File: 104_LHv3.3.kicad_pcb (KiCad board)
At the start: 2 copper layers, 437.8 x 130.6 mm, 241 parts, among them K1 CHRY_MX, K10 CHRY_MX, K100 CHRY_MX, K101 CHRY_MX, K102 CHRY_MX, K103 CHRY_MX, K104 CHRY_MX, K11 CHRY_MX, K12 CHRY_MX, K13 CHRY_MX, K14 CHRY_MX, K15 CHRY_MX, K16 CHRY_MX, K17 CHRY_MX, K18 CHRY_MX, K19 CHRY_MX, K2 CHRY_MX, K20 CHRY_MX, K21 CHRY_MX, K22 CHRY_MX, K23 CHRY_MX, K24 CHRY_MX, K25 CHRY_MX, K26 CHRY_MX, K27 CHRY_MX, K28 CHRY_MX, K29 CHRY_MX, K3 CHRY_MX, K30 CHRY_MX, K31 CHRY_MX, K32 CHRY_MX, K33 CHRY_MX, K34 CHRY_MX, K35 CHRY_MX, K36 CHRY_MX, K37 CHRY_MX, K38 CHRY_MX, K39 CHRY_MX, K4 CHRY_MX, K40 CHRY_MX, K41 CHRY_MX, K42 CHRY_MX, K43 CHRY_MX, K44 CHRY_MX, K45 CHRY_MX, K46 CHRY_MX, K47 CHRY_MX, K48 CHRY_MX, K49 CHRY_MX, K5 CHRY_MX, K50 CHRY_MX, K51 CHRY_MX, K52 CHRY_MX, K53 CHRY_MX, K54 CHRY_MX, K55 CHRY_MX, K56 CHRY_MX, K57 CHRY_MX, K58 CHRY_MX, K59 CHRY_MX, K6 CHRY_MX, K60 CHRY_MX, K61 CHRY_MX, K62 CHRY_MX, K63 CHRY_MX, K64 CHRY_MX, K65 CHRY_MX, K66 CHRY_MX, K67 CHRY_MX, K68 CHRY_MX, K69 CHRY_MX, K7 CHRY_MX, K70 CHRY_MX, K71 CHRY_MX, K72 CHRY_MX, K73 CHRY_MX, K74 CHRY_MX, K75 CHRY_MX, K76 CHRY_MX, K77 CHRY_MX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

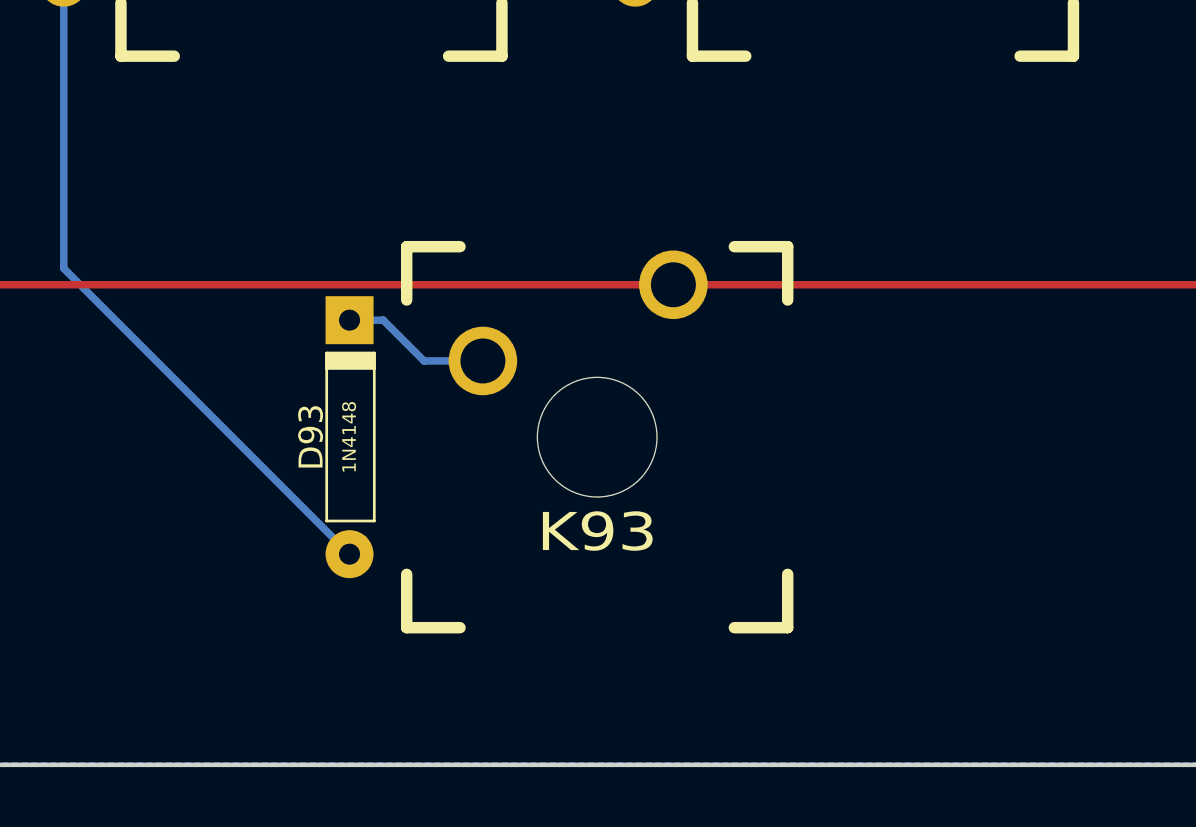
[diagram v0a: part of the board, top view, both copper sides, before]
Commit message: Tweaks in Stabs
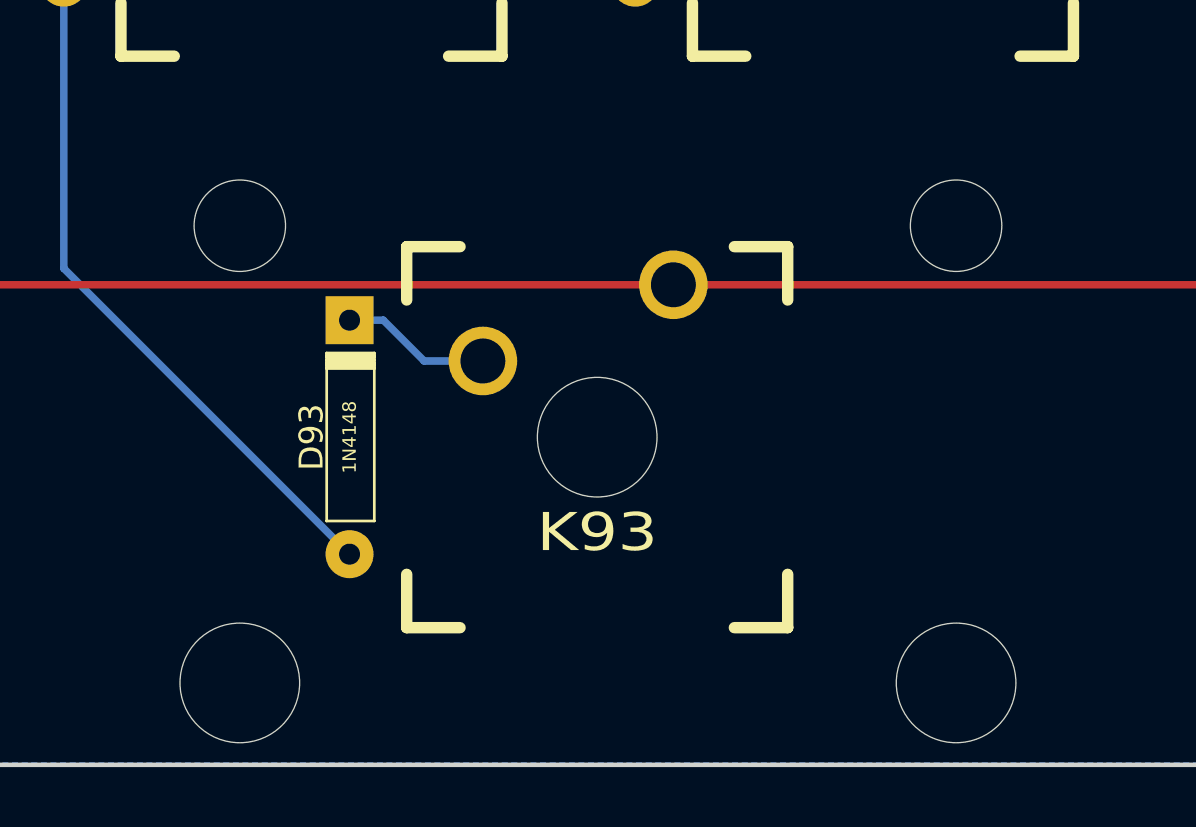
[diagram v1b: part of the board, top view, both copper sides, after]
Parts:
- added 2.0u: 2.0u, mx_stabs:Mx_Stab_200, F.Cu at (116.2, 197.4)
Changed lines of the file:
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@@
     (tracks 1560)
     (zones 0)
-    (modules 241)
+    (modules 242)
     (nets 159)
   )
@@
     (add_net /VCC)
   )
+  (module mx_stabs:Mx_Stab_200 (layer F.Cu)
+    (at 116.2304 197.4215)
+    (descr MXALPS)
+    (tags MXALPS)
+    (fp_text reference 2.0u (at 0 10.5) (layer B.SilkS)
+      (effects (font (size 1 1) (thickness 0.2)) (justify mirror))
+    )
+    (fp_text value 2.0u (at 14.732 10.668) (layer B.SilkS) hide
+      (effects (font (size 1.524 1.524) (thickness 0.3048)) (justify mirror))
+    )
+    (fp_line (start -18.923 -9.398) (end 18.923 -9.398) (layer Dwgs.User) (width 0.1524))
+    (fp_line (start 18.923 -9.398) (end 18.923 9.398) (layer Dwgs.User) (width 0.1524))
+    (fp_line (start 18.923 9.398) (end -18.923 9.398) (layer Dwgs.User) (width 0.1524))
+    (fp_line (start -18.923 9.398) (end -18.923 -9.398) (layer Dwgs.User) (width 0.1524))
+    (fp_line (start -6.985 -6.985) (end 6.985 -6.985) (layer Eco2.User) (width 0.1524))
+    (fp_line (start 6.985 -6.985) (end 6.985 -4.8768) (layer Eco2.User) (width 0.1524))
+    (fp_line (start 6.985 -4.8768) (end 8.6106 -4.8768) (layer Eco2.User) (width 0.1524))
+    (fp_line (start 8.6106 -4.8768) (end 8.6106 -5.6896) (layer Eco2.User) (width 0.1524))
+    (fp_line (start 8.6106 -5.6896) (end 15.2654 -5.6896) (layer Eco2.User) (width 0.1524))
+    (fp_line (start 15.2654 -5.6896) (end 15.2654 -2.286) (layer Eco2.User) (width 0.1524))
+    (fp_line (start 15.2654 -2.286) (end 16.129 -2.286) (layer Eco2.User) (width 0.1524))
+    (fp_line (start 16.129 -2.286) (end 16.129 0.508) (layer Eco2.User) (width 0.1524))
+    (fp_line (start 16.129 0.508) (end 15.2654 0.508) (layer Eco2.User) (width 0.1524))
+    (fp_line (start 15.2654 0.508) (end 15.2654 6.604) (layer Eco2.User) (width 0.1524))
+    (fp_line (start 15.2654 6.604) (end 14.224 6.604) (layer Eco2.User) (width 0.1524))
+    (fp_line (start 14.224 6.604) (end 14.224 7.7724) (layer Eco2.User) (width 0.1524))
+    (fp_line (start 14.224 7.7724) (end 9.652 7.7724) (layer Eco2.User) (width 0.1524))
+    (fp_line (start 9.652 7.7724) (end 9.652 6.604) (layer Eco2.User) (width 0.1524))
+    (fp_line (start 9.652 6.604) (end 8.6106 6.604) (layer Eco2.User) (width 0.1524))
+    (fp_line (start 8.6106 6.604) (end 8.6106 5.8166) (layer Eco2.User) (width 0.1524))
+    (fp_line (start 8.6106 5.8166) (end 6.985 5.8166) (layer Eco2.User) (width 0.1524))
+    (fp_line (start 6.985 5.8166) (end 6.985 6.985) (layer Eco2.User) (width 0.1524))
+    (fp_line (start 6.985 6.985) (end -6.985 6.985) (layer Eco2.User) (width 0.1524))
+    (fp_line (start -6.985 6.985) (end -6.985 5.8166) (layer Eco2.User) (width 0.1524))
+    (fp_line (start -6.985 5.8166) (end -8.6106 5.8166) (layer Eco2.User) (width 0.1524))
+    (fp_line (start -8.6106 5.8166) (end -8.6106 6.604) (layer Eco2.User) (width 0.1524))
+    (fp_line (start -8.6106 6.604) (end -9.652 6.604) (layer Eco2.User) (width 0.1524))
+    (fp_line (start -9.652 6.604) (end -9.652 7.7724) (layer Eco2.User) (width 0.1524))
+    (fp_line (start -9.652 7.7724) (end -14.224 7.7724) (layer Eco2.User) (width 0.1524))
+    (fp_line (start -14.224 7.7724) (end -14.224 6.604) (layer Eco2.User) (width 0.1524))
+    (fp_line (start -14.224 6.604) (end -15.2654 6.604) (layer Eco2.User) (width 0.1524))
+    (fp_line (start -15.2654 6.604) (end -15.2654 0.508) (layer Eco2.User) (width 0.1524))
+    (fp_line (start -15.2654 0.508) (end -16.129 0.508) (layer Eco2.User) (width 0.1524))
+    (fp_line (start -16.129 0.508) (end -16.129 -2.286) (layer Eco2.User) (width 0.1524))
+    (fp_line (start -16.129 -2.286) (end -15.2654 -2.286) (layer Eco2.User) (width 0.1524))
+    (fp_line (start -15.2654 -2.286) (end -15.2654 -5.6896) (layer Eco2.User) (width 0.1524))
+    (fp_line (start -15.2654 -5.6896) (end -8.6106 -5.6896) (layer Eco2.User) (width 0.1524))
+    (fp_line (start -8.6106 -5.6896) (end -8.6106 -4.8768) (layer Eco2.User) (width 0.1524))
+    (fp_line (start -8.6106 -4.8768) (end -6.985 -4.8768) (layer Eco2.User) (width 0.1524))
+    (fp_line (start -6.985 -4.8768) (end -6.985 -6.985) (layer Eco2.User) (width 0.1524))
+    (fp_line (start 15.367 -7.62) (end 8.509 -7.62) (layer Cmts.User) (width 0.1524))
+    (fp_line (start 8.509 -7.62) (end 8.509 7.62) (layer Cmts.User) (width 0.1524))
+    (fp_line (start 8.509 7.62) (end -8.509 7.62) (layer Cmts.User) (width 0.1524))
+    (fp_line (start -8.509 7.62) (end -8.509 -7.62) (layer Cmts.User) (width 0.1524))
+    (fp_line (start -8.509 -7.62) (end -15.367 -7.62) (layer Cmts.User) (width 0.1524))
+    (fp_line (start -15.367 -7.62) (end -15.367 10.16) (layer Cmts.User) (width 0.1524))
+    (fp_line (start -15.367 10.16) (end 15.367 10.16) (layer Cmts.User) (width 0.1524))
+    (fp_line (start 15.367 10.16) (end 15.367 -7.62) (layer Cmts.User) (width 0.1524))
+    (fp_line (start 7.75 6.4) (end 7.75 -6.4) (layer Dwgs.User) (width 0.3))
+    (fp_line (start -7.62 -7.62) (end 7.62 -7.62) (layer Dwgs.User) (width 0.3))
+    (fp_line (start 7.62 -7.62) (end 7.62 7.62) (layer Dwgs.User) (width 0.3))
+    (fp_line (start 7.62 7.62) (end -7.62 7.62) (layer Dwgs.User) (width 0.3))
+    (fp_line (start -7.62 7.62) (end -7.62 -7.62) (layer Dwgs.User) (width 0.3))
+    (pad "" np_thru_hole circle (at -11.938 -6.985) (size 3.048 3.048) (drill 3.048) (layers *.Cu *.Mask))
+    (pad "" np_thru_hole circle (at 11.938 -6.985) (size 3.048 3.048) (drill 3.048) (layers *.Cu *.Mask))
+    (pad "" np_thru_hole circle (at -11.938 8.255) (size 3.9878 3.9878) (drill 3.9878) (layers *.Cu *.Mask))
+    (pad "" np_thru_hole circle (at 11.938 8.255) (size 3.9878 3.9878) (drill 3.9878) (layers *.Cu *.Mask))
+  )
   (module logo:kilogo (layer F.Cu)
